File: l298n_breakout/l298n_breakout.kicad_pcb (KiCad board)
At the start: 2 copper layers, 36.4 x 34.9 mm, 17 parts, among them J1 Conn_01x03_Male, J14 M0, J2 M1, M0 Conn_01x03_Male, U1 L293E

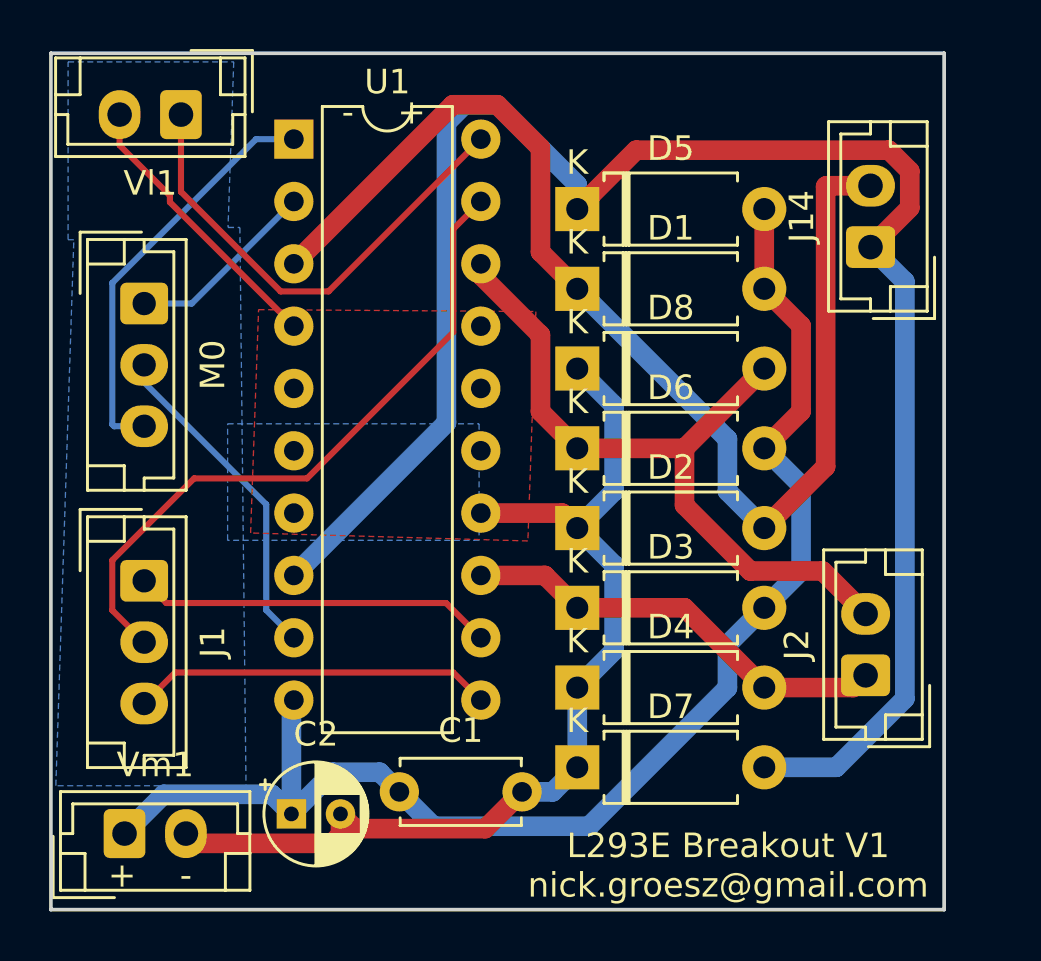
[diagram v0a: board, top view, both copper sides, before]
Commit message: L298N breakout
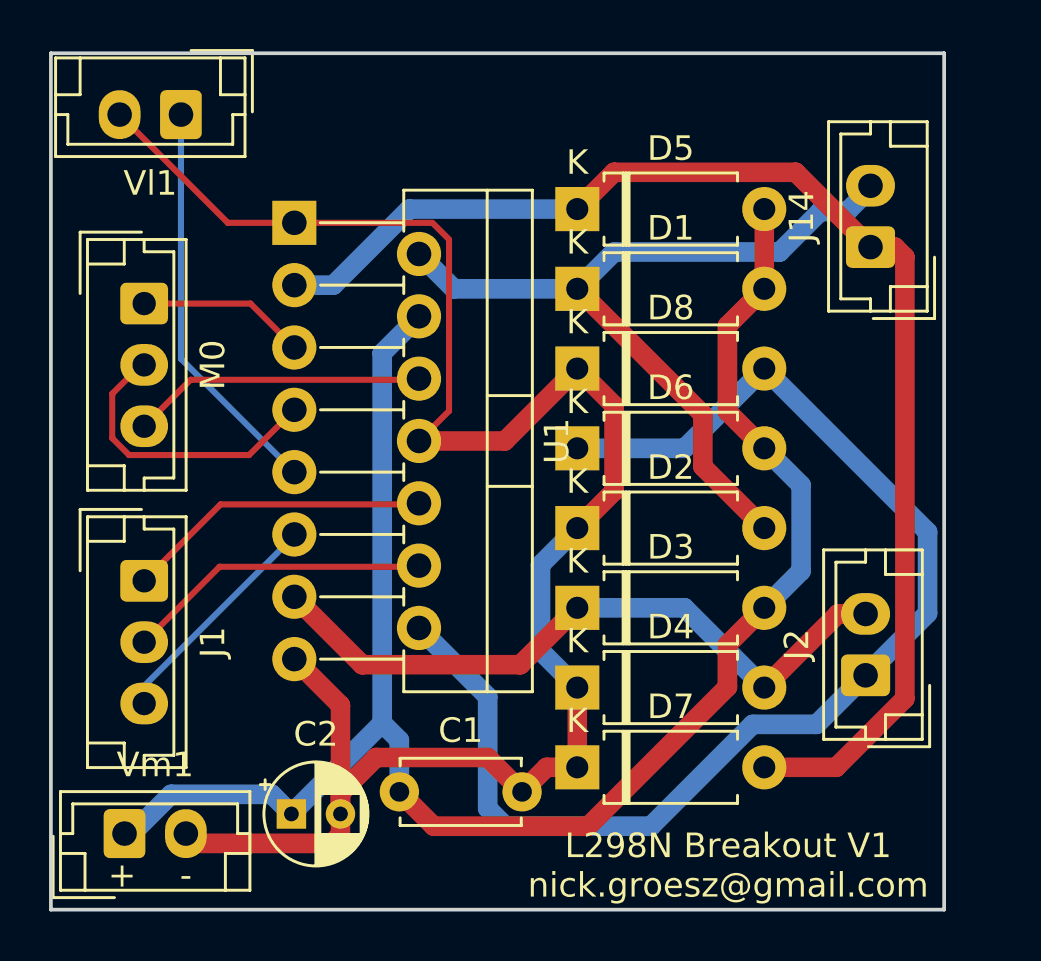
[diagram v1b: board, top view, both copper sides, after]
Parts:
- U1: value L293E -> L298HN; footprint Package_DIP:DIP-20_W7.62mm -> Package_TO_SOT_THT:TO-220-15_P2.54x2.54mm_StaggerOdd_Lead4.58mm_Vertical
- moved U1 3.41 mm to (92.2, 64.3), turned to 270 degrees
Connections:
- J2 pad 1: Net-(D3-Pad1) -> Net-(D6-Pad1)
- J2 pad 2: Net-(D6-Pad1) -> Net-(D3-Pad1)
- U1 pad 1: Net-(M0-Pad3) -> /GND
- U1 pad 10: Net-(C1-Pad1) -> Net-(J1-Pad1)
- U1 pad 12: Net-(J1-Pad1) -> Net-(J1-Pad2)
- U1 pad 14: /GND -> Net-(D6-Pad1)
- U1 pad 2: Net-(M0-Pad1) -> Net-(D1-Pad1)
- U1 pad 3: Net-(D1-Pad1) -> Net-(D5-Pad1)
- U1 pad 4: /GND -> Net-(C1-Pad1)
- U1 pad 5: /GND -> Net-(M0-Pad1)
- U1 pad 6: /GND -> Net-(M0-Pad3)
- U1 pad 7: /GND -> Net-(M0-Pad2)
- U1 pad 8: Net-(D5-Pad1) -> /GND
- U1 pad 9: Net-(M0-Pad2) -> Net-(U1-Pad9)
- Vl1 pad 1: Net-(U1-Pad20) -> Net-(U1-Pad9)
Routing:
- net /GND: track 52.9 -> 77.3 mm
- net Net-(D6-Pad1): track 29.6 -> 52.0 mm
- net Net-(D5-Pad1): track 73.5 -> 53.1 mm
- net Net-(U1-Pad20): track 19.6 -> 0.00 mm
- net Net-(U1-Pad9): track 0.00 -> 16.5 mm
- net Net-(D1-Pad1): track 49.5 -> 33.7 mm
- net Net-(C1-Pad1): track 56.8 -> 72.2 mm
- net Net-(J1-Pad2): track 27.4 -> 12.5 mm
- net Net-(D3-Pad1): track 17.8 -> 28.0 mm
- net Net-(J1-Pad3): track 14.7 -> 9.42 mm
- net Net-(M0-Pad3): track 16.9 -> 12.0 mm
- net Net-(J1-Pad1): track 14.7 -> 12.5 mm
- net Net-(M0-Pad2): track 13.6 -> 12.1 mm
- net Net-(M0-Pad1): track 7.82 -> 6.86 mm
- removed copper zone on B.Cu, net /GND
- removed copper zone on F.Cu, net /GND
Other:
- board text added: "L298N Breakout V1 nick.groesz@gmail.com"
- board text removed: "L293E Breakout V1 nick.groesz@gmail.com"
